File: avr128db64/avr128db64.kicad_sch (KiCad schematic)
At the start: 16 parts, among them J1 BUS1, J7 47571-0001, U1 AVR128DB64x-xPT, U2 MCP7940N-xSN, U3 74HCT138, U5 74HCT574, U6 74HCT257, U7 AS6C4008-55PCN, Y1 32kHz

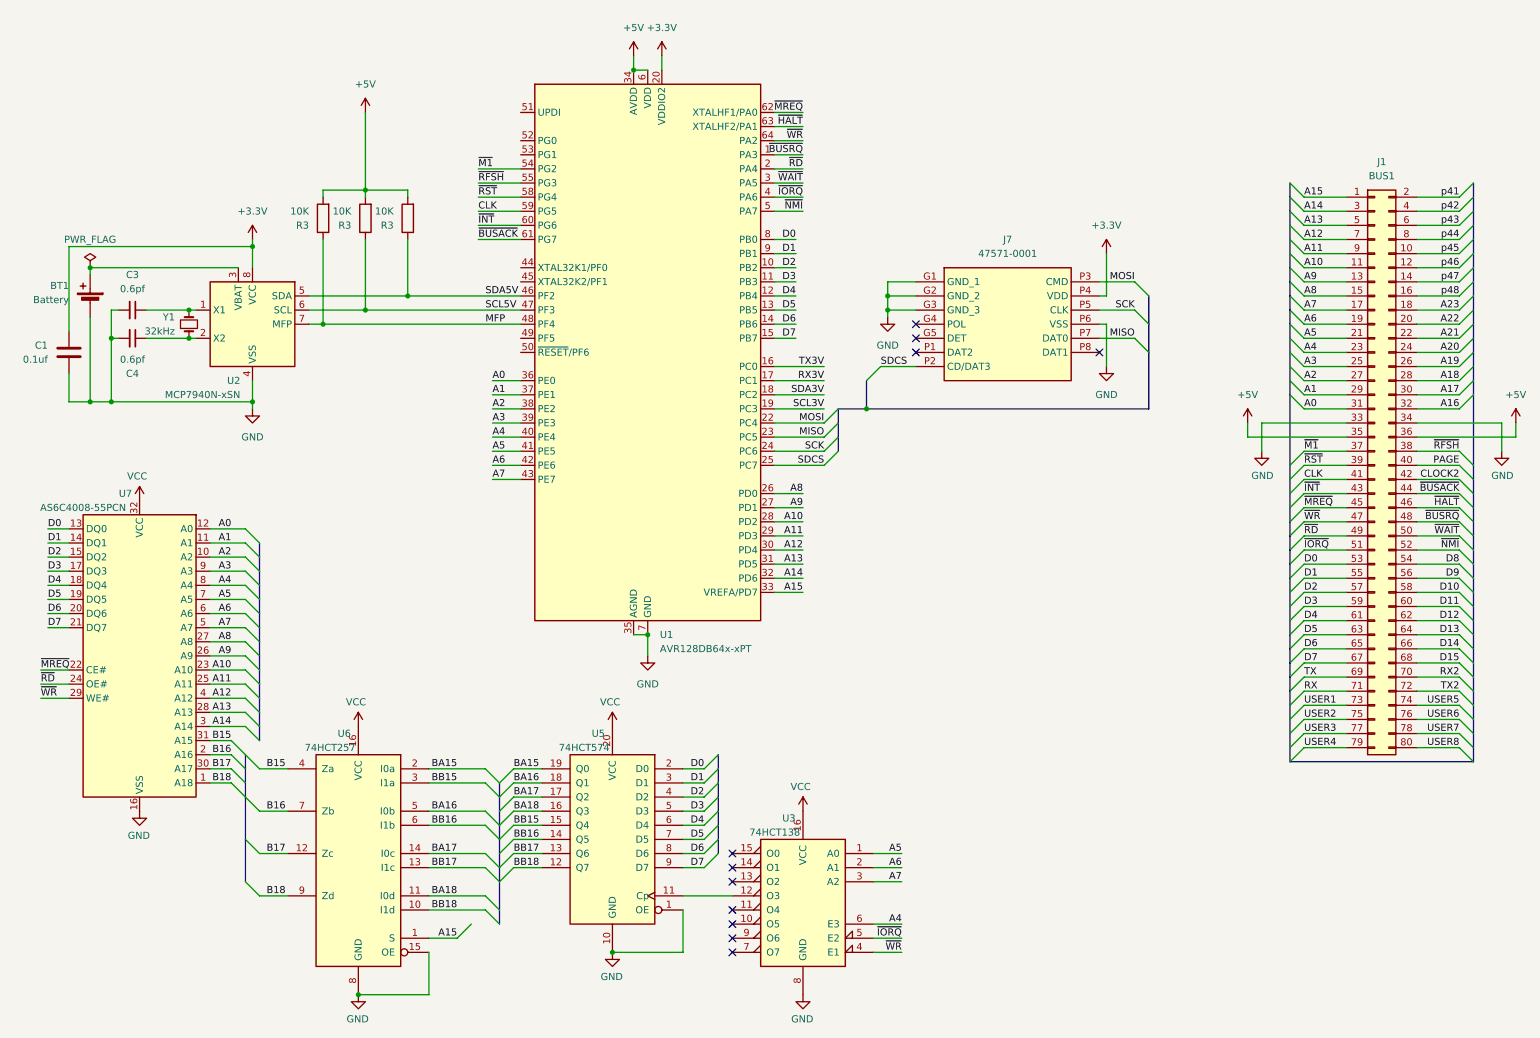
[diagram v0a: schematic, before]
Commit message: Further updates to PCB
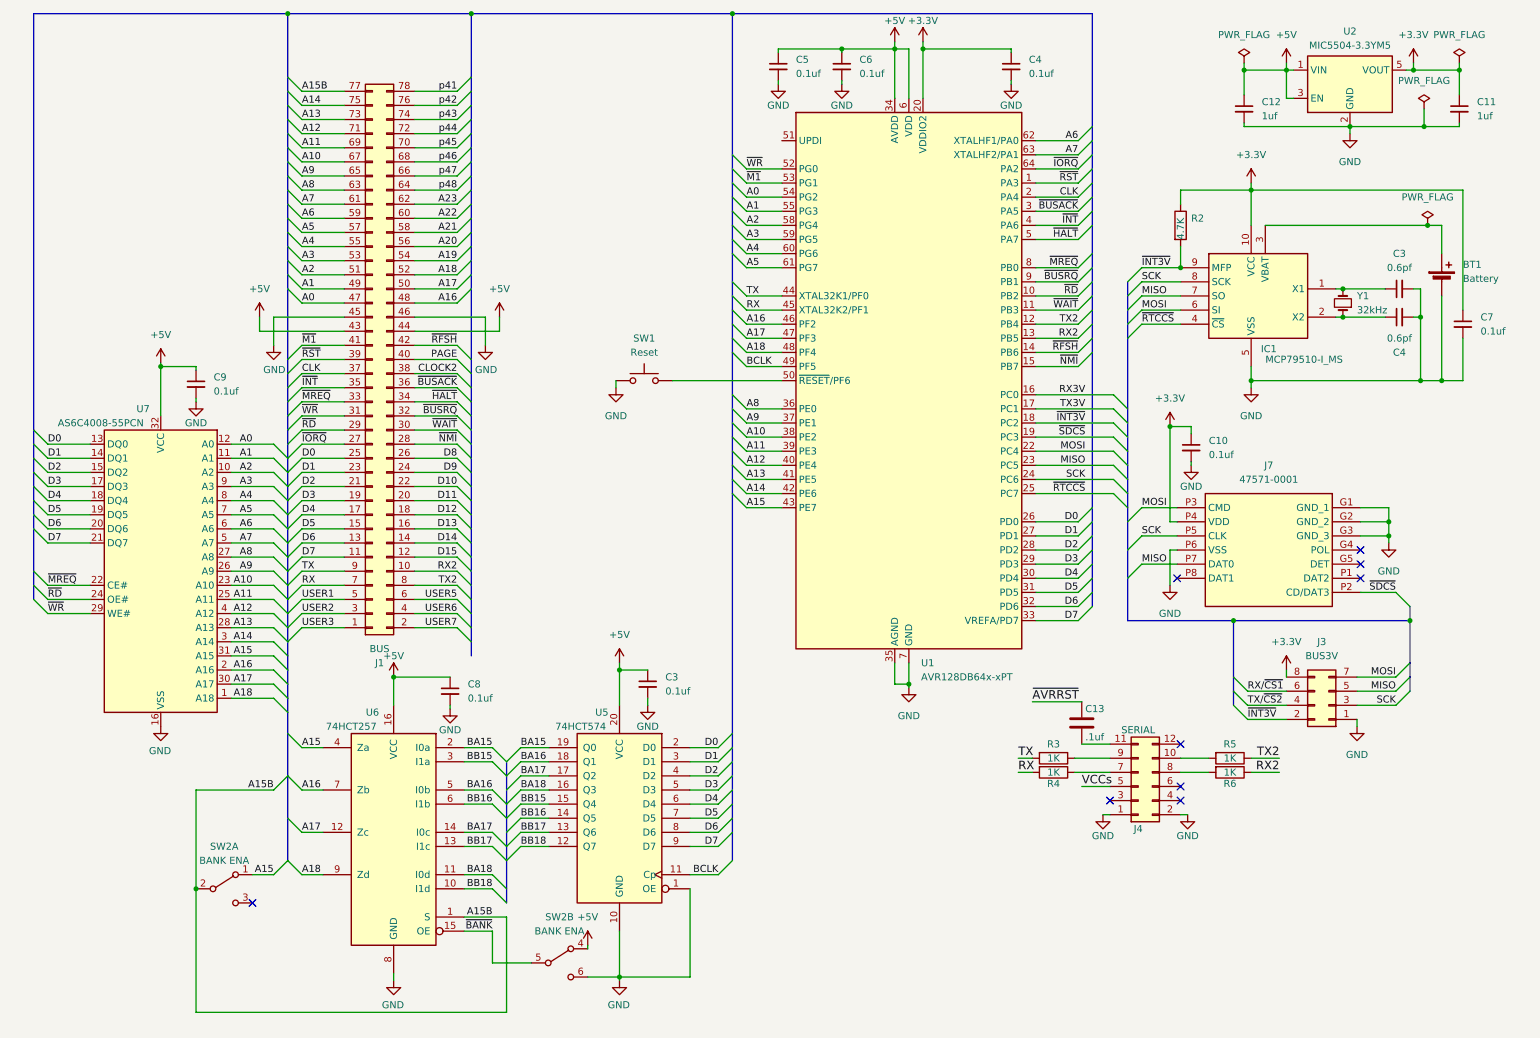
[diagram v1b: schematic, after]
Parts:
- removed C1: 0.1uf, Capacitor_SMD:C_0603_1608Metric, symbol Device:C
- removed J1: BUS1, Connector_PinSocket_2.54mm:PinSocket_2x40_P2.54mm_Vertical, symbol Connector_Generic:Conn_02x40_Odd_Even
- removed R3 (x3): 10K, Resistor_SMD:R_0201_0603Metric, symbol Device:R
- removed U2: MCP7940N-xSN, Package_SO:SOIC-8_3.9x4.9mm_P1.27mm, symbol Timer_RTC:MCP7940N-xSN
- removed U3: 74HCT138, Package_SO:SO-16_3.9x9.9mm_P1.27mm, symbol 74xx:74LS138
- added C10, C3, C4, C5, C6, C7, C8, C9: 0.1uf, Capacitor_SMD:C_0201_0603Metric, symbol Device:C_Small
- added C11, C12: 1uf, Capacitor_SMD:C_0201_0603Metric, symbol Device:C_Small
- added C13: .1uf, Capacitor_SMD:C_0201_0603Metric, symbol Device:C
- added IC1: MCP79510-I_MS, SamacSys_Parts:SOP50P490X110-10N, symbol SamacSys_Parts:MCP79510-I_MS
- added J1: BUS, Connector_PinHeader_2.54mm:PinHeader_2x39_P2.54mm_Horizontal, symbol Connector_Generic:Conn_02x39_Odd_Even
- added J3: BUS3V, Connector_PinHeader_2.54mm:PinHeader_2x04_P2.54mm_Horizontal, symbol Connector_Generic:Conn_02x04_Odd_Even
- added J4: SERIAL, Connector_PinHeader_2.54mm:PinHeader_2x06_P2.54mm_Horizontal, symbol Connector_Generic:Conn_02x06_Odd_Even
- added R2: 4.7K, Resistor_SMD:R_0201_0603Metric, symbol Device:R
- added R3, R4, R5, R6: 1K, Resistor_SMD:R_0201_0603Metric, symbol Device:R
- added SW1: Reset, Button_Switch_THT:SW_PUSH_6mm, symbol Switch:SW_Push
- added SW2: BANK ENA, SamacSys_Parts:JS202011SCQN, symbol Switch:SW_DPDT_x2
- added U2: MIC5504-3.3YM5, Package_TO_SOT_SMD:SOT-23-5, symbol Regulator_Linear:MIC5504-3.3YM5
- U5: footprint Package_SO:SO-20_12.8x7.5mm_P1.27mm -> Package_SO:SOIC-20W_7.5x12.8mm_P1.27mm
- U7: footprint Package_SO:SSOP-32_11.305x20.495mm_P1.27mm -> Package_SO:TSOP-I-32_18.4x8mm_P0.5mm
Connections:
- net B15 is gone; now on net A15: U6.4 (Za), U7.31 (A15)
- net B16 is gone; now on net A16: U6.7 (Zb), U7.2 (A16)
- net B17 is gone; now on net A17: U6.12 (Zc), U7.30 (A17)
- net B18 is gone; now on net A18: U6.9 (Zd), U7.1 (A18)
- net MFP is gone; now on net A18: U1.48 (PF4)
- net SCL5V is gone; now on net A17: U1.47 (PF3)
- net SDA5V is gone; now on net A16: U1.46 (PF2)
- net VCC is gone; now on net +5V: U5.20 (VCC), U6.16 (VCC), U7.32 (VCC)
- net +3.3V: now also C10.1, C11.1, C4.1, C7.1, IC1.10 (VCC), J3.8 (Pin_8), R2.1, U2.5 (VOUT)
- net +5V: now also C12.1, C3.1, C5.1, C6.1, C8.1, C9.1, J1.43 (Pin_43), J1.44 (Pin_44), SW2.4 (A), U2.1 (VIN), U2.3 (EN)
- net A0: now also U1.54 (PG2), J1.47 (Pin_47); no longer U1.36 (PE0)
- net A1: now also U1.55 (PG3), J1.49 (Pin_49); no longer U1.37 (PE1)
- net A10: now also U1.38 (PE2), J1.67 (Pin_67); no longer U1.28 (PD2)
- net A11: now also U1.39 (PE3), J1.69 (Pin_69); no longer U1.29 (PD3)
- net A12: now also U1.40 (PE4), J1.71 (Pin_71); no longer U1.30 (PD4)
- net A13: now also U1.41 (PE5), J1.73 (Pin_73); no longer U1.31 (PD5)
- net A14: now also U1.42 (PE6), J1.75 (Pin_75); no longer U1.32 (PD6)
- net A15: now also U1.43 (PE7), SW2.1 (A); no longer U1.33 (VREFA/PD7), U6.1 (S)
- net A16: now also J1.48 (Pin_48)
- net A17: now also J1.50 (Pin_50)
- net A18: now also J1.52 (Pin_52)
- net A19: now also J1.54 (Pin_54)
- net A2: now also U1.58 (PG4), J1.51 (Pin_51); no longer U1.38 (PE2)
- net A20: now also J1.56 (Pin_56)
- net A21: now also J1.58 (Pin_58)
- net A22: now also J1.60 (Pin_60)
- net A23: now also J1.62 (Pin_62)
- net A3: now also U1.59 (PG5), J1.53 (Pin_53); no longer U1.39 (PE3)
- net A4: now also U1.60 (PG6), J1.55 (Pin_55); no longer U1.40 (PE4)
- net A5: now also U1.61 (PG7), J1.57 (Pin_57); no longer U1.41 (PE5)
- net A6: now also U1.62 (XTALHF1/PA0), J1.59 (Pin_59); no longer U1.42 (PE6)
- net A7: now also U1.63 (XTALHF2/PA1), J1.61 (Pin_61); no longer U1.43 (PE7)
- net A8: now also U1.36 (PE0), J1.63 (Pin_63); no longer U1.26 (PD0)
- net A9: now also U1.37 (PE1), J1.65 (Pin_65); no longer U1.27 (PD1)
- net CLK: now also U1.2 (PA4), J1.37 (Pin_37); no longer U1.59 (PG5)
- net CLOCK2: now also J1.38 (Pin_38)
- net D0: now also U1.26 (PD0), J1.25 (Pin_25); no longer U1.8 (PB0)
- net D1: now also U1.27 (PD1), J1.23 (Pin_23); no longer U1.9 (PB1)
- net D10: now also J1.22 (Pin_22)
- net D11: now also J1.20 (Pin_20)
- net D12: now also J1.18 (Pin_18)
- net D13: now also J1.16 (Pin_16)
- net D14: now also J1.14 (Pin_14)
- net D15: now also J1.12 (Pin_12)
- net D2: now also U1.28 (PD2), J1.21 (Pin_21); no longer U1.10 (PB2)
- net D3: now also U1.29 (PD3), J1.19 (Pin_19); no longer U1.11 (PB3)
- net D4: now also U1.30 (PD4), J1.17 (Pin_17); no longer U1.12 (PB4)
- net D5: now also U1.31 (PD5), J1.15 (Pin_15); no longer U1.13 (PB5)
- net D6: now also U1.32 (PD6), J1.13 (Pin_13); no longer U1.14 (PB6)
- net D7: now also U1.33 (VREFA/PD7), J1.11 (Pin_11); no longer U1.15 (PB7)
- net D8: now also J1.26 (Pin_26)
- net D9: now also J1.24 (Pin_24)
- net GND: now also C10.2, C11.2, C12.2, C3.2, C4.2, C5.2, C6.2, C7.2, C8.2, C9.2, IC1.5 (VSS), J1.45 (Pin_45), J1.46 (Pin_46), J3.1 (Pin_1), J4.1 (Pin_1), J4.2 (Pin_2), SW1.1, SW2.6 (C), U2.2 (GND); no longer U6.15 (OE)
- net MISO: now also IC1.7 (SO), J3.5 (Pin_5)
- net MOSI: now also IC1.6 (SI), J3.7 (Pin_7)
- net PAGE: now also J1.40 (Pin_40)
- net RX: now also U1.45 (XTAL32K2/PF1), J1.7 (Pin_7), R4.2
- net RX2: now also U1.13 (PB5), J1.10 (Pin_10), R6.1
- net RX3V: now also U1.16 (PC0); no longer U1.17 (PC1)
- net SCK: now also IC1.8 (SCK), J3.3 (Pin_3)
- net TX: now also U1.44 (XTAL32K1/PF0), J1.9 (Pin_9), R3.2
- net TX2: now also U1.12 (PB4), J1.8 (Pin_8), R5.1
- net TX3V: now also U1.17 (PC1); no longer U1.16 (PC0)
- net USER1: now also J1.5 (Pin_5)
- net USER2: now also J1.3 (Pin_3)
- net USER3: now also J1.1 (Pin_1)
- net USER5: now also J1.6 (Pin_6)
- net USER6: now also J1.4 (Pin_4)
- net USER7: now also J1.2 (Pin_2)
- net p41: now also J1.78 (Pin_78)
- net p42: now also J1.76 (Pin_76)
- net p43: now also J1.74 (Pin_74)
- net p44: now also J1.72 (Pin_72)
- net p45: now also J1.70 (Pin_70)
- net p46: now also J1.68 (Pin_68)
- net p47: now also J1.66 (Pin_66)
- net p48: now also J1.64 (Pin_64)
- net ~{BUSACK}: now also U1.3 (PA5), J1.36 (Pin_36); no longer U1.61 (PG7)
- net ~{BUSRQ}: now also U1.9 (PB1), J1.32 (Pin_32); no longer U1.1 (PA3)
- net ~{HALT}: now also U1.5 (PA7), J1.34 (Pin_34); no longer U1.63 (XTALHF2/PA1)
- net ~{INT}: now also U1.4 (PA6), J1.35 (Pin_35); no longer U1.60 (PG6)
- net ~{IORQ}: now also U1.64 (PA2), J1.27 (Pin_27); no longer U1.4 (PA6)
- net ~{M1}: now also U1.53 (PG1), J1.41 (Pin_41); no longer U1.54 (PG2)
- net ~{MREQ}: now also U1.8 (PB0), J1.33 (Pin_33); no longer U1.62 (XTALHF1/PA0)
- net ~{NMI}: now also U1.15 (PB7), J1.28 (Pin_28); no longer U1.5 (PA7)
- net ~{RD}: now also U1.10 (PB2), J1.29 (Pin_29); no longer U1.2 (PA4)
- net ~{RFSH}: now also U1.14 (PB6), J1.42 (Pin_42); no longer U1.55 (PG3)
- net ~{RST}: now also U1.1 (PA3), J1.39 (Pin_39); no longer U1.58 (PG4)
- net ~{WAIT}: now also U1.11 (PB3), J1.30 (Pin_30); no longer U1.3 (PA5)
- net ~{WR}: now also U1.52 (PG0), J1.31 (Pin_31); no longer U1.64 (PA2)
- net at C4.1, Y1.1: now also IC1.2 (X2)
- net BCLK: now reaches U5.11 (Cp)
- net BCLK: now also U1.49 (PF5)
- net at C3.1, Y1.2: now also IC1.1 (X1)
- net at U1.50 (~{RESET}/PF6): now also SW1.2
- net at BT1.1 (+): now also IC1.3 (VBAT)
- net SCL3V renamed ~{SDCS}
- net ~{SDCS}: now also J7.P2 (CD/DAT3)
- net SDA3V renamed ~{INT3V}
- net ~{INT3V}: now also IC1.9 (MFP), J3.2 (Pin_2), R2.2
- net SDCS renamed ~{RTCCS}
- net ~{RTCCS}: now also IC1.4 (~{CS}); no longer J7.P2 (CD/DAT3)
- new net: C13.2, J4.11 (Pin_11)
- new net: J4.7 (Pin_7), R4.1
- new net: J4.10 (Pin_10), R5.2
- new net: J4.8 (Pin_8), R6.2
- new net: J4.9 (Pin_9), R3.1
- new net A15B: J1.77 (Pin_77), SW2.2 (B), U6.1 (S)
- new net RX/~{CS1}: J3.6 (Pin_6)
- new net TX/~{CS2}: J3.4 (Pin_4)
- new net VCCs: J4.5 (Pin_5)
- new net ~{AVRRST}: C13.1
- new net ~{BANK}: SW2.5 (B), U6.15 (OE)
- no-connect marks 11 -> 9
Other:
- moved on the sheet: BT1, C3, C4, J7, U1, U5, U6, U7, Y1
